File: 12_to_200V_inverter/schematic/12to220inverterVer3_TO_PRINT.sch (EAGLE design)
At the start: 255 parts, among them IC1 UC3842, IC10 TL494, IC2 PC817, IC3 LM358, IC4 TL431, IC5 LM317, IC6 74HC595, IC7 74HC595, IC8 ATTINY45, IC9 TL431, J100 0, J101 0, J2 0, J3 0, T10 16N60, T11 BC847, T12 BC847, T13 AO3401, T14 AO3401, T15 BC847, T16 BSS84, T17 BC847, T18 BC847, T19 BSS84, T2 IRF830, T21 BC847, T22 BC847, T23 BSS84, T24 BC847, T3 IRF830, T4 BC847, T5 BC857, T6 BC857, T7 IRFZ24N, T8 IRFZ24N, T9 BC857, U100 DF06S, X1 BAT+, X2 LAMP1, X3 LAMP1, X4 BAT-, X5 220VAC, X6 LAMP1_SWITCH, X7 LAMP1_SWITCH, X8 MCU_PROGRAMMING

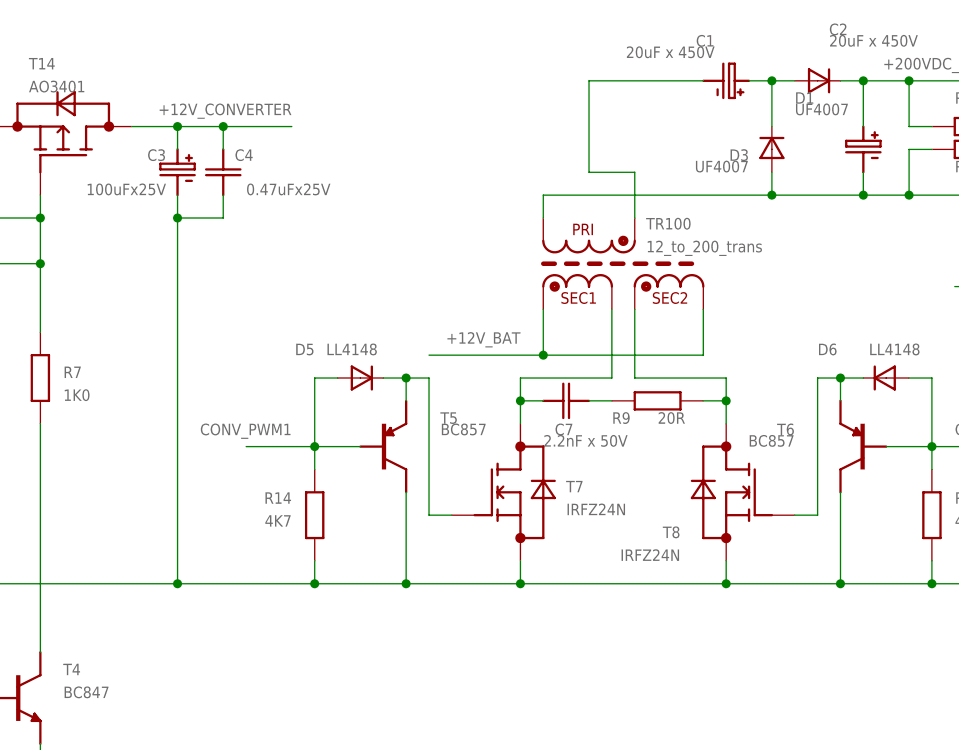
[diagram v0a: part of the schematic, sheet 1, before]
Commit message: 12 to 200V inverter. Timny changes to schematic and board.
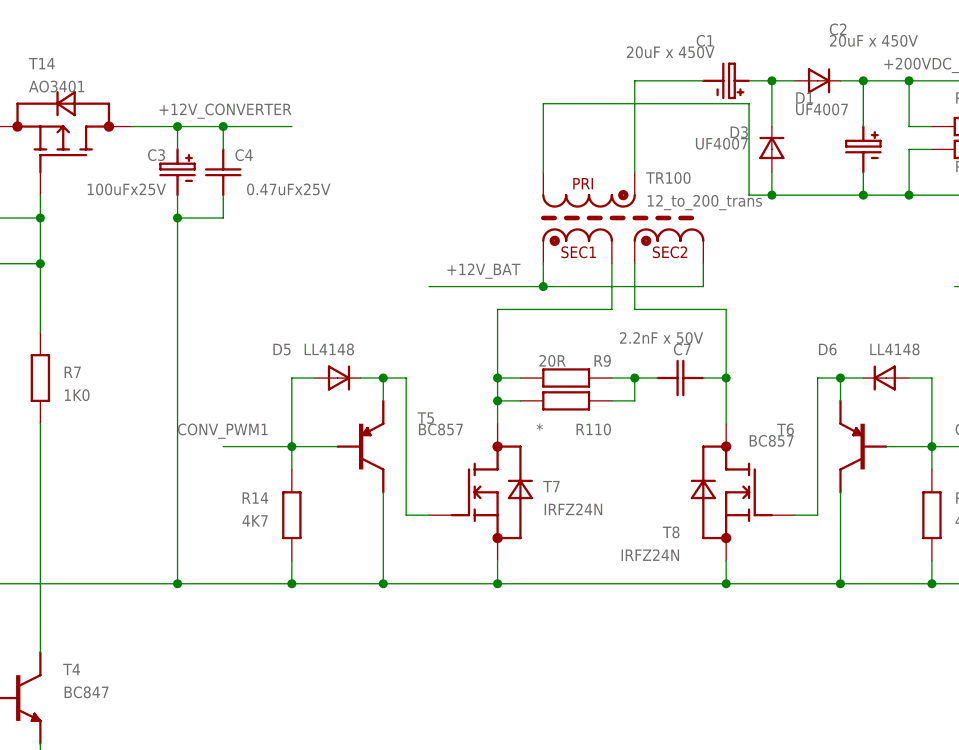
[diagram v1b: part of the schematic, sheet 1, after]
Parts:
- added R110: *, __MyCommonLib1:RSMD_1206
- F2: device __MyCommonLib1:FUSE20X5.6MM -> __MyCommonLib1:FUSE(20X5MM_VERT_WIRE)
- IC4: device __MyCommonLib1:TL431TO-92A_PINS_SWAPPED -> __MyCommonLib1:TL431TO-92A
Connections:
- net N$24: now also R110.PIN0, R9.PIN0; no longer C7.PIN1
- net N$25: now also C7.PIN1; no longer R9.PIN0
- net N$26: now also R110.PIN1
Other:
- moved on the sheet: C7, D5, R14, R9, T5, T7, TR100
